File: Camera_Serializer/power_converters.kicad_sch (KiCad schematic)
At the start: 36 parts, among them Q1 BSS138, Q2 BSS138, U3 TPS62133RGTR, U4 TPS62131RGTT, U5 TPS73601DBVR, U6 MIC5528-3.3YMT-TR

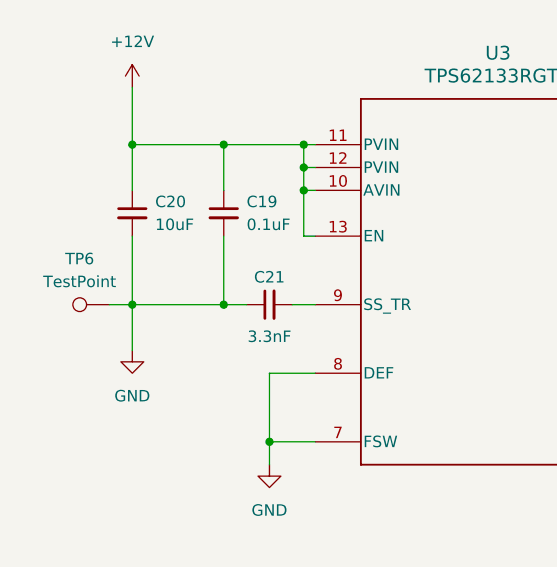
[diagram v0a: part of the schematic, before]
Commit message: Finished routing
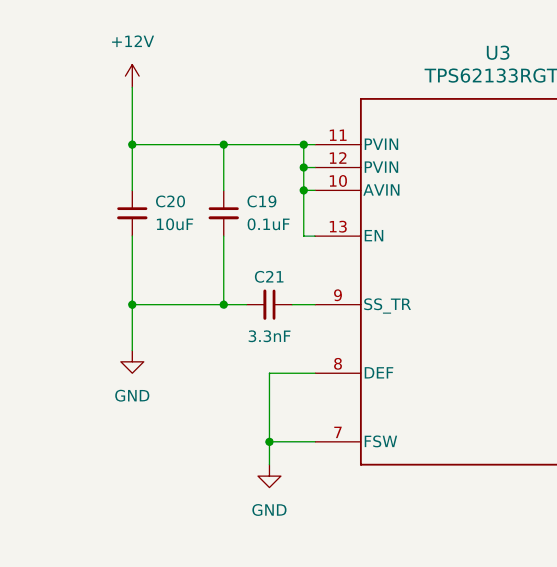
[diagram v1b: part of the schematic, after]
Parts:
- removed TP6: TestPoint, TestPoint:TestPoint_Pad_D1.0mm, symbol Connector:TestPoint
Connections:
- net GND: now also C21.2; no longer C21.1
- net at U3.9 (SS_TR): now also C21.1; no longer C21.2
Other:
- moved on the sheet: C21
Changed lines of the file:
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@@
-	(wire
-		(pts
-			(xy 25.4 57.15) (xy 22.86 57.15)
-		)
-		(stroke
-			(width 0)
-			(type default)
-		)
-	)
 	(wire
 		(pts
@@
 	)
 	(symbol
-		(lib_id "Connector:TestPoint")
-		(at 22.86 57.15 90)
-		(unit 1)
-		(exclude_from_sim no)
-		(in_bom yes)
-		(on_board yes)
-		(dnp no)
-		(fields_autoplaced yes)
-		(property "Reference" "TP6"
-			(at 19.558 52.07 90)
-			(effects
-				(font
-					(size 1.27 1.27)
-				)
-			)
-		)
-		(property "Value" "TestPoint"
-			(at 19.558 54.61 90)
-			(effects
-				(font
-					(size 1.27 1.27)
-				)
-			)
-		)
-		(property "Footprint" "TestPoint:TestPoint_Pad_D1.0mm"
-			(at 22.86 52.07 0)
-			(effects
-				(font
-					(size 1.27 1.27)
-				)
-				(hide yes)
-			)
-		)
-		(property "Datasheet" "~"
-			(at 22.86 52.07 0)
-			(effects
-				(font
-					(size 1.27 1.27)
-				)
-				(hide yes)
-			)
-		)
-		(property "Description" "test point"
-			(at 22.86 57.15 0)
-			(effects
-				(font
-					(size 1.27 1.27)
-				)
-				(hide yes)
-			)
-		)
-		(pin "1"
-		)
-		(instances
-			(project "Camera_serializer"
-				(path "/ebaf1619-da94-4b8e-b57a-a386470e666e/aa1b48ff-d467-42b0-a250-5333a1eca37c"
-					(reference "TP6")
-					(unit 1)
-				)
-			)
-		)
-	)
-	(symbol
 		(lib_id "power:+3V3")
 		(at 171.45 120.65 0)
@@
 	(symbol
 		(lib_id "Device:C_Small")
-		(at 40.64 57.15 90)
-		(unit 1)
-		(exclude_from_sim no)
+		(at 40.64 57.15 270)
+		(mirror x)
+		(unit 1)
+		(exclude_from_sim no)
